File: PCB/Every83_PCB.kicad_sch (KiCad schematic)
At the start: 36 parts, among them IC2 GD25Q16, J1 781710004, J3 SM03B-SRSS-TB, J4 SM03B-SRSS-TB, Q3 DMG2305, SW101 KMR2, SW102 KMR2, U2 AP2112(3.3V), U3 MCP73831T-2ACI/OT, X3 JSTPH, Y2 32.768

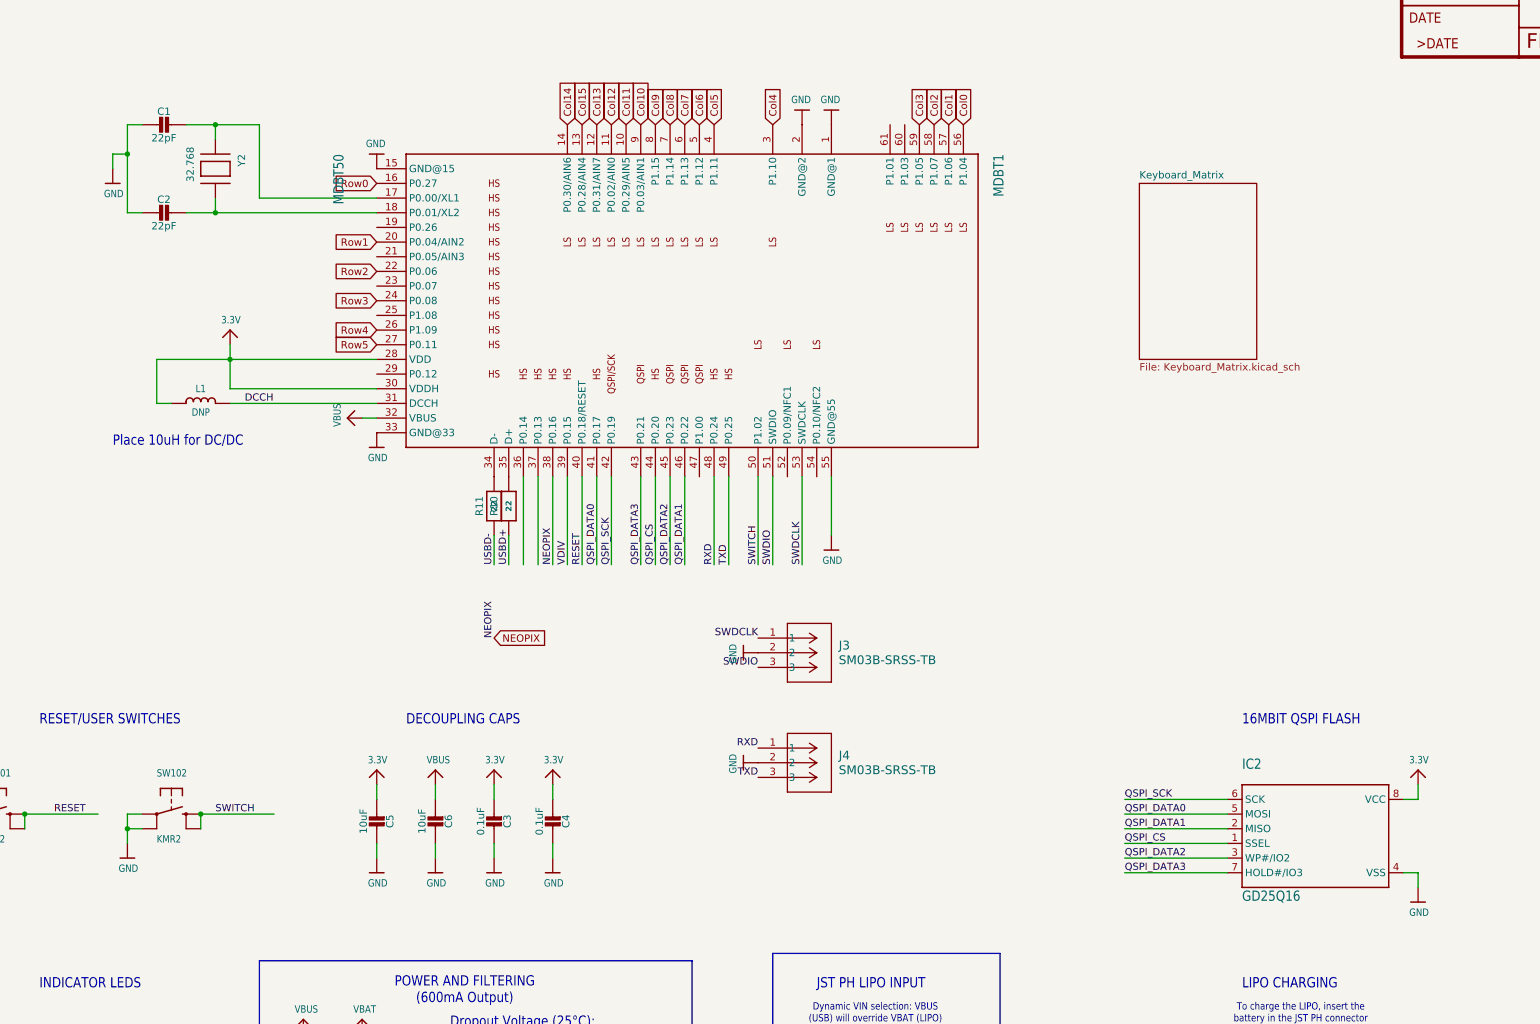
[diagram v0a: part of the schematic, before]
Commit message: swap micro
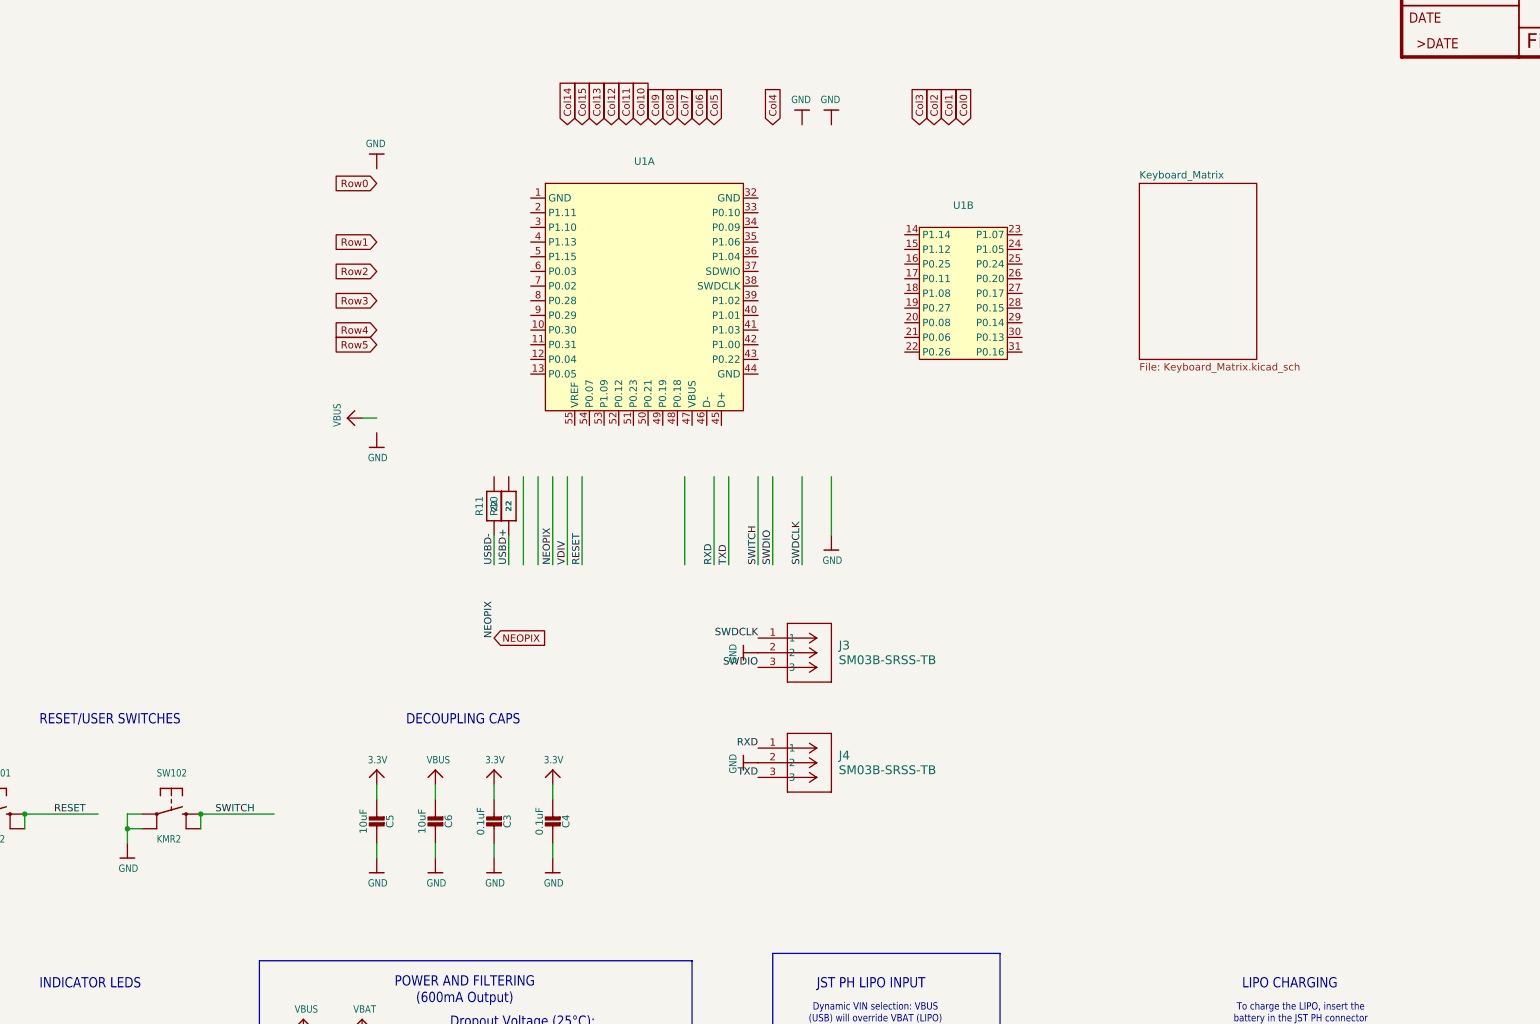
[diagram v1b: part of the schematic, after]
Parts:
- removed C1, C2: 22pF, Adafruit nRF52840 Bluefruit Feather Express Rev D:0603-NO, symbol Adafruit nRF52840 Bluefruit Feather Express Rev D-eagle-import:CAP_CERAMIC0603_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
- removed IC2: GD25Q16, Adafruit nRF52840 Bluefruit Feather Express Rev D:USON8, symbol Adafruit nRF52840 Bluefruit Feather Express Rev D-eagle-import:SPIFLASH_8PINUX
- removed L1: DNP, Adafruit nRF52840 Bluefruit Feather Express Rev D:_0805MP, symbol Adafruit nRF52840 Bluefruit Feather Express Rev D-eagle-import:INDUCTOR_0805MP
- removed MDBT1: MDBT50, Adafruit nRF52840 Bluefruit Feather Express Rev D:MDBT50, symbol Adafruit nRF52840 Bluefruit Feather Express Rev D-eagle-import:MDBT50
- removed Y2: 32.768, Adafruit nRF52840 Bluefruit Feather Express Rev D:XTAL3215, symbol Adafruit nRF52840 Bluefruit Feather Express Rev D-eagle-import:XTAL-3.2X1.5
- added U1: ~, symbol JohnDeere:Core52480
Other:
- note removed: "16MBIT QSPI FLASH"
- note removed: "Place 10uH for DC/DC"
